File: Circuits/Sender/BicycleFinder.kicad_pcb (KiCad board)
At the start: 2 copper layers, 64.1 x 40.1 mm, 12 parts, among them P1 WRITER-VCC, SW1 SW_PUSH, SW2 REED SW, U1 TWE_LITE_SMD, U2 HN2S01FU

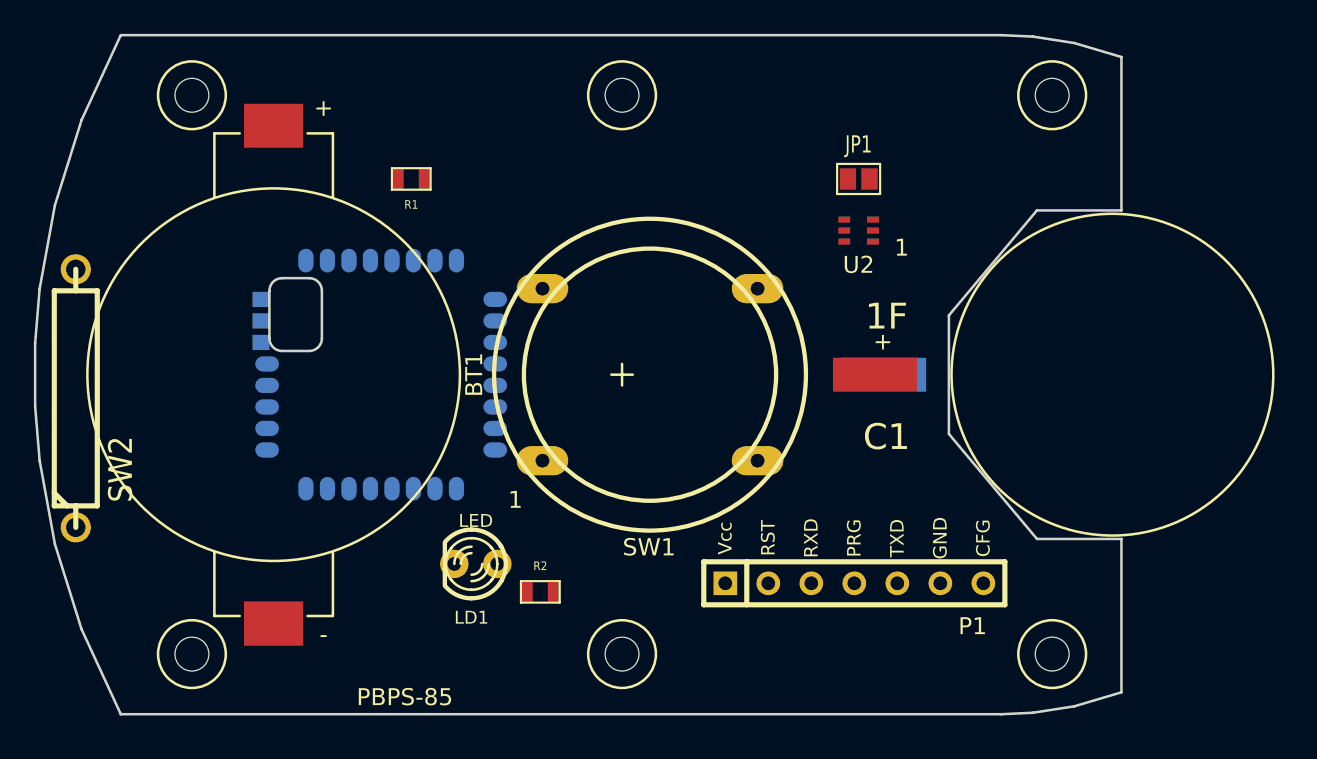
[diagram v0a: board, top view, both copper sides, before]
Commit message: Reviewing connections.
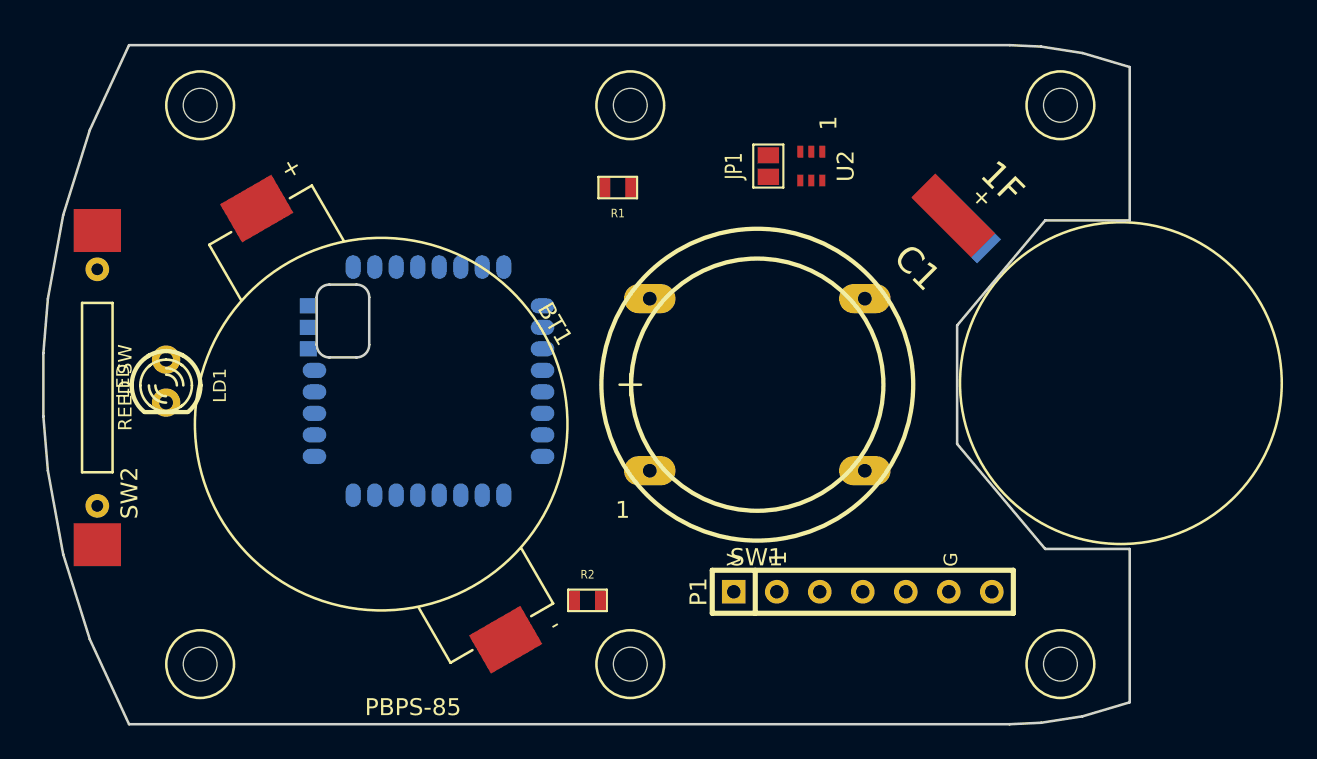
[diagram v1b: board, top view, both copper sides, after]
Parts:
- SW2: footprint R6 -> REEDSW
- moved LD1 21.2 mm to (21.6, 34.3), turned to 270 degrees
- moved R1 12.2 mm to (48.3, 22.9)
- moved BT1 6.99 mm to (34.3, 36.8), turned to 300 degrees
- moved SW1 6.36 mm to (56.5, 34.5)
- moved JP1 5.39 mm to (57.1, 21.6), turned to 0 degrees
- moved U2 4.72 mm to (59.7, 21.6), turned to 270 degrees
- moved R2 2.83 mm to (46.5, 47.2)
- moved U1 2.82 mm to (37.1, 34.3)
- moved SW2 1.42 mm to (17.5, 34.7)
- moved PBPS-85 0.77 mm to (49.0, 34.5)
- moved C1 0.71 mm to (78.0, 34.4), turned to 135 degrees
- moved P1 0.71 mm to (62.7, 46.7)
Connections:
- net N-0000016 renamed /STOP
- net N-0000017 renamed /WUP
- P1 pad 1: N-000001 -> N-0000013
- P1 pad 2: N-0000012 -> N-000005
- P1 pad 3: N-000005 -> N-0000012
- P1 pad 4: N-0000014 -> N-0000018
- P1 pad 5: N-0000019 -> GND
- P1 pad 6: GND -> N-0000014
- U1 pad 12: N-0000013 -> N-0000014
- U1 pad 2: N-0000014 -> N-0000012
- U1 pad 21: N-0000012 -> N-0000013
- U1 pad 8: N-0000019 -> N-0000018
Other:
- outline, holes or cut-outs redrawn
